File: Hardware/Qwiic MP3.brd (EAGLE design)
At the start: 25.4 x 50.8 mm, 97 parts, among them J1 MICRO-SD, J3 PTH, J7 ISP, J8 3.5mm Audio, J9 Poke-Home, U1 TPA2005D1, U2 WT2003S, U3 AP2112-3.3V, U4 ATTINY84-ARDUINO

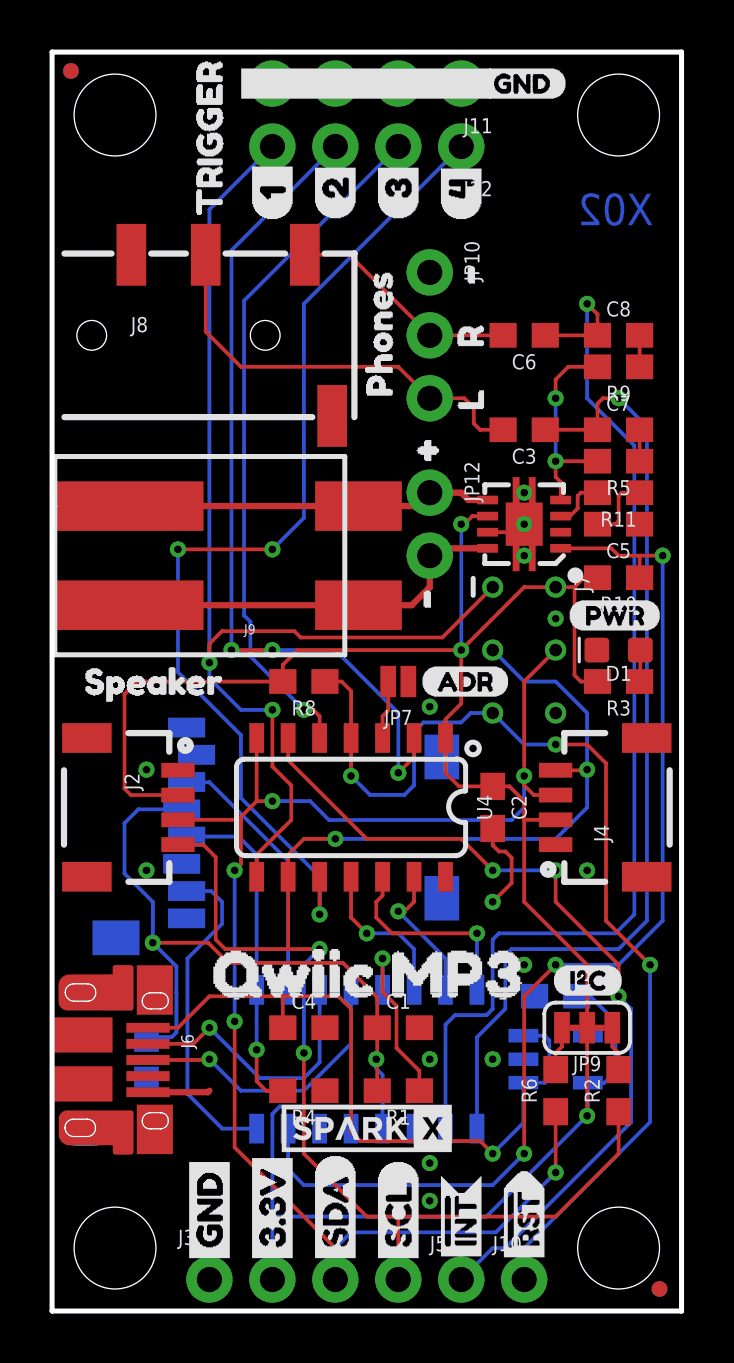
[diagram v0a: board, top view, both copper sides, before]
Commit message: Nearing production code
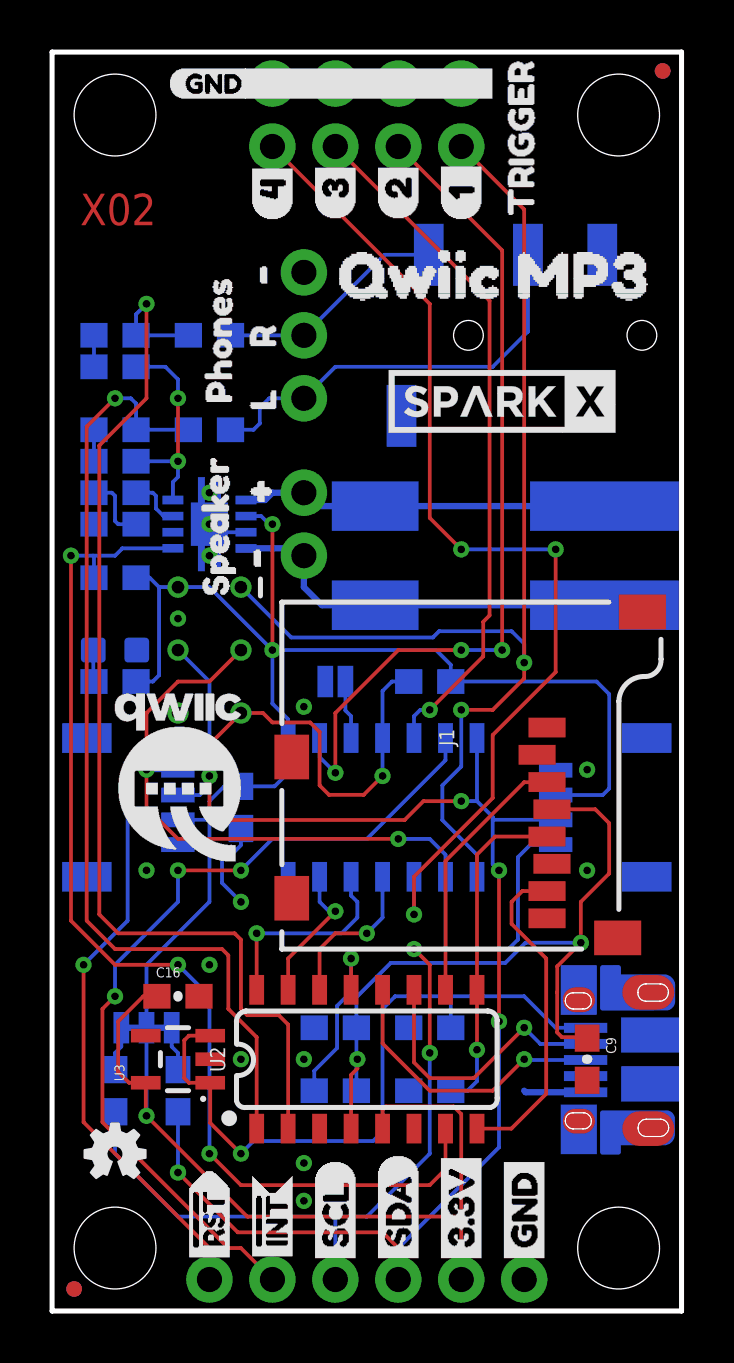
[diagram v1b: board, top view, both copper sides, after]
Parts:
- C3, C6: value 10uF -> 0.22uF
- moved FRAME1 66.0 mm to (45.7, -17.8), flipped to the bottom
- moved J8 25.4 mm to (25.4, 39.4), flipped to the bottom
- moved U$20 24.6 mm to (25.0, 25.4), flipped to the bottom
- moved JP1 23.9 mm to (24.6, 50.0), flipped to the top
- moved JP6 23.9 mm to (24.6, 50.0), flipped to the bottom
- moved JP2 23.6 mm to (0.89, 0.89), flipped to the bottom
- moved JP5 23.6 mm to (0.89, 0.89), flipped to the top
- moved C5 20.3 mm to (2.54, 31.8), flipped to the bottom
- moved C7 20.3 mm to (2.54, 35.6), flipped to the bottom
- moved C8 20.3 mm to (2.54, 39.4), flipped to the bottom
- moved D1 20.3 mm to (2.54, 26.7), flipped to the bottom
- moved J6 20.3 mm to (22.9, 10.2), flipped to the bottom
- moved JP11 20.3 mm to (22.9, 2.54), flipped to the bottom
- moved JP13 20.3 mm to (2.54, 2.54), flipped to the bottom
- moved JP3 20.3 mm to (22.9, 48.3), flipped to the bottom
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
